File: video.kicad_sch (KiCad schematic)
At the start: 4 parts, among them J2 Board Interconnect Female, J2 Video Output Female, J3 Conn_02x08_Odd_Even

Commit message: move to samx4
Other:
- company: (none) -> Dragon Data
- title: (none) -> Dragon 32 CPU UK PAL
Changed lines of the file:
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@@
   (paper "A3")
   (title_block
+    (title "Dragon 32 CPU UK PAL")
     (date "2023-05-25")
     (rev "3.0")
-    (comment 2 "Reposition dram and buffer")
+    (company "Dragon Data")
+    (comment 1 "Modified by Julian Brown")
+    (comment 2 "SAMx4 by Ciaran Anscomb")
   )
   (no_connect (at 167.64 168.91))

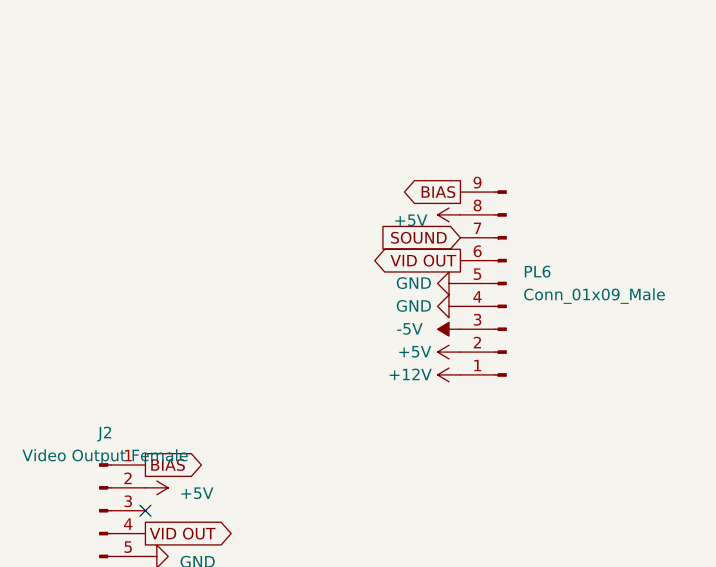
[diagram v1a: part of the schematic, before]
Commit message: serial wiring
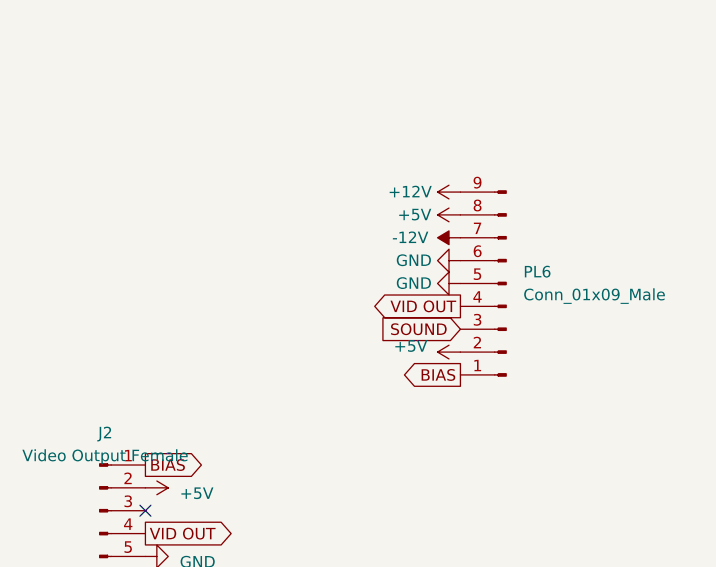
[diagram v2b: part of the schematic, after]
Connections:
- net +12V: now also PL6.9 (Pin_9); no longer PL6.1 (Pin_1)
- net -5V: no longer PL6.3 (Pin_3)
- net BIAS: now also PL6.1 (Pin_1); no longer PL6.9 (Pin_9)
- net GND: now also PL6.6 (Pin_6); no longer PL6.4 (Pin_4)
- net SOUND: now also PL6.3 (Pin_3); no longer PL6.7 (Pin_7)
- net VID OUT: now also PL6.4 (Pin_4); no longer PL6.6 (Pin_6)
- new net -12V: PL6.7 (Pin_7)
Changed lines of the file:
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@@
     )
   )
-  (global_label "VID OUT" (shape output) (at 202.6412 141.1224 180) (fields_autoplaced)
-    (effects (font (size 1.27 1.27)) (justify right))
-    (property "Intersheetrefs" "${INTERSHEET_REFS}" (at 193.0356 141.1224 0)
+  (global_label "VID OUT" (shape output) (at 202.6412 146.2024 180) (fields_autoplaced)
+    (effects (font (size 1.27 1.27)) (justify right))
+    (property "Intersheetrefs" "${INTERSHEET_REFS}" (at 193.0356 146.2024 0)
       (effects (font (size 1.27 1.27)) (justify right) hide)
     )
@@
     )
   )
-  (global_label "SOUND" (shape input) (at 202.6412 138.5824 180) (fields_autoplaced)
-    (effects (font (size 1.27 1.27)) (justify right))
-    (property "Intersheetrefs" "${INTERSHEET_REFS}" (at 193.9186 138.5824 0)
+  (global_label "SOUND" (shape input) (at 202.6412 148.7424 180) (fields_autoplaced)
+    (effects (font (size 1.27 1.27)) (justify right))
+    (property "Intersheetrefs" "${INTERSHEET_REFS}" (at 193.9186 148.7424 0)
       (effects (font (size 1.27 1.27)) (justify right) hide)
     )
@@
     )
   )
-  (global_label "BIAS" (shape output) (at 202.6412 133.5024 180) (fields_autoplaced)
-    (effects (font (size 1.27 1.27)) (justify right))
-    (property "Intersheetrefs" "${INTERSHEET_REFS}" (at 196.2167 133.5024 0)
+  (global_label "BIAS" (shape output) (at 202.6412 153.8224 180) (fields_autoplaced)
+    (effects (font (size 1.27 1.27)) (justify right))
+    (property "Intersheetrefs" "${INTERSHEET_REFS}" (at 196.2167 153.8224 0)
       (effects (font (size 1.27 1.27)) (justify right) hide)
     )
@@
     )
   )
-  (symbol (lib_id "power:GND") (at 202.6412 146.2024 270) (unit 1)
-    (in_bom yes) (on_board yes) (dnp no) (fields_autoplaced)
-    (property "Reference" "#PWR019" (at 196.2912 146.2024 0)
-      (effects (font (size 1.27 1.27)) hide)
-    )
-    (property "Value" "GND" (at 199.4662 146.2023 90)
+  (symbol (lib_id "power:GND") (at 202.6412 141.1224 270) (mirror x) (unit 1)
+    (in_bom yes) (on_board yes) (dnp no) (fields_autoplaced)
+    (property "Reference" "#PWR019" (at 196.2912 141.1224 0)
+      (effects (font (size 1.27 1.27)) hide)
+    )
+    (property "Value" "GND" (at 199.4662 141.1225 90)
       (effects (font (size 1.27 1.27)) (justify right))
     )
-    (property "Footprint" "" (at 202.6412 146.2024 0)
-      (effects (font (size 1.27 1.27)) hide)
-    )
-    (property "Datasheet" "" (at 202.6412 146.2024 0)
+    (property "Footprint" "" (at 202.6412 141.1224 0)
+      (effects (font (size 1.27 1.27)) hide)
+    )
+    (property "Datasheet" "" (at 202.6412 141.1224 0)
       (effects (font (size 1.27 1.27)) hide)
     )
@@
     )
   )
-  (symbol (lib_id "power:+5V") (at 202.6412 151.2824 90) (unit 1)
+  (symbol (lib_id "power:+5V") (at 202.6412 136.0424 90) (mirror x) (unit 1)
     (in_bom yes) (on_board yes) (dnp no)
-    (property "Reference" "#PWR0281" (at 206.4512 151.2824 0)
-      (effects (font (size 1.27 1.27)) hide)
-    )
-    (property "Value" "+5V" (at 195.6562 151.2824 90)
+    (property "Reference" "#PWR0281" (at 206.4512 136.0424 0)
+      (effects (font (size 1.27 1.27)) hide)
+    )
+    (property "Value" "+5V" (at 195.6562 136.0424 90)
       (effects (font (size 1.27 1.27)) (justify right))
     )
+    (property "Footprint" "" (at 202.6412 136.0424 0)
+      (effects (font (size 1.27 1.27)) hide)
+    )
+    (property "Datasheet" "" (at 202.6412 136.0424 0)
+      (effects (font (size 1.27 1.27)) hide)
+    )
+    (pin "1")
+    (instances
+      (project "Dragon32"
+        (path "/0c3dceba-7c95-4b3d-b590-0eb581444beb/d9dba8db-e731-4cb4-b2de-fefd65b288bc"
+          (reference "#PWR0281") (unit 1)
+        )
+      )
+    )
+  )
+  (symbol (lib_id "power:+5V") (at 202.6412 151.2824 90) (mirror x) (unit 1)
+    (in_bom yes) (on_board yes) (dnp no) (fields_autoplaced)
+    (property "Reference" "#PWR052" (at 206.4512 151.2824 0)
+      (effects (font (size 1.27 1.27)) hide)
+    )
+    (property "Value" "+5V" (at 198.9836 150.6474 90)
+      (effects (font (size 1.27 1.27)) (justify left))
+    )
     (property "Footprint" "" (at 202.6412 151.2824 0)
       (effects (font (size 1.27 1.27)) hide)
     )
     (property "Datasheet" "" (at 202.6412 151.2824 0)
-      (effects (font (size 1.27 1.27)) hide)
-    )
-    (pin "1")
-    (instances
-      (project "Dragon32"
-        (path "/0c3dceba-7c95-4b3d-b590-0eb581444beb/d9dba8db-e731-4cb4-b2de-fefd65b288bc"
-          (reference "#PWR0281") (unit 1)
-        )
-      )
-    )
-  )
-  (symbol (lib_id "power:+5V") (at 202.6412 136.0424 90) (unit 1)
-    (in_bom yes) (on_board yes) (dnp no) (fields_autoplaced)
-    (property "Reference" "#PWR052" (at 206.4512 136.0424 0)
-      (effects (font (size 1.27 1.27)) hide)
-    )
-    (property "Value" "+5V" (at 198.9836 136.6774 90)
-      (effects (font (size 1.27 1.27)) (justify left))
-    )
-    (property "Footprint" "" (at 202.6412 136.0424 0)
-      (effects (font (size 1.27 1.27)) hide)
-    )
-    (property "Datasheet" "" (at 202.6412 136.0424 0)
       (effects (font (size 1.27 1.27)) hide)
     )
@@
     )
   )
+  (symbol (lib_id "power:-12V") (at 202.6412 138.5824 90) (unit 1)
+    (in_bom yes) (on_board yes) (dnp no) (fields_autoplaced)
+    (property "Reference" "#PWR095" (at 200.1012 138.5824 0)
+      (effects (font (size 1.27 1.27)) hide)
+    )
+    (property "Value" "-12V" (at 199.0852 138.5824 90)
+      (effects (font (size 1.27 1.27)) (justify left))
+    )
+    (property "Footprint" "" (at 202.6412 138.5824 0)
+      (effects (font (size 1.27 1.27)) hide)
+    )
+    (property "Datasheet" "" (at 202.6412 138.5824 0)
+      (effects (font (size 1.27 1.27)) hide)
+    )
+    (pin "1")
+    (instances
+      (project "Dragon32"
+        (path "/0c3dceba-7c95-4b3d-b590-0eb581444beb/d9dba8db-e731-4cb4-b2de-fefd65b288bc"
+          (reference "#PWR095") (unit 1)
+        )
+      )
+    )
+  )
   (symbol (lib_id "power:GND") (at 137.1092 167.9448 90) (unit 1)
     (in_bom yes) (on_board yes) (dnp no) (fields_autoplaced)
@@
     )
   )
-  (symbol (lib_id "power:-5V") (at 202.6412 148.7424 90) (unit 1)
-    (in_bom yes) (on_board yes) (dnp no)
-    (property "Reference" "#PWR0282" (at 200.1012 148.7424 0)
-      (effects (font (size 1.27 1.27)) hide)
-    )
-    (property "Value" "-5V" (at 195.5292 148.7424 90)
-      (effects (font (size 1.27 1.27)) (justify right))
-    )
-    (property "Footprint" "" (at 202.6412 148.7424 0)
-      (effects (font (size 1.27 1.27)) hide)
-    )
-    (property "Datasheet" "" (at 202.6412 148.7424 0)
-      (effects (font (size 1.27 1.27)) hide)
-    )
-    (pin "1")
-    (instances
-      (project "Dragon32"
-        (path "/0c3dceba-7c95-4b3d-b590-0eb581444beb/d9dba8db-e731-4cb4-b2de-fefd65b288bc"
-          (reference "#PWR0282") (unit 1)
-        )
-      )
-    )
-  )
-  (symbol (lib_id "power:GND") (at 202.6412 143.6624 270) (unit 1)
+  (symbol (lib_id "power:GND") (at 202.6412 143.6624 270) (mirror x) (unit 1)
     (in_bom yes) (on_board yes) (dnp no) (fields_autoplaced)
     (property "Reference" "#PWR018" (at 196.2912 143.6624 0)
       (effects (font (size 1.27 1.27)) hide)
     )
-    (property "Value" "GND" (at 199.4662 143.6623 90)
+    (property "Value" "GND" (at 199.4662 143.6625 90)
       (effects (font (size 1.27 1.27)) (justify right))
     )
@@
     )
   )
-  (symbol (lib_id "power:+12V") (at 202.6412 153.8224 90) (unit 1)
-    (in_bom yes) (on_board yes) (dnp no) (fields_autoplaced)
-    (property "Reference" "#PWR022" (at 206.4512 153.8224 0)
-      (effects (font (size 1.27 1.27)) hide)
-    )
-    (property "Value" "+12V" (at 199.4662 153.8223 90)
+  (symbol (lib_id "power:+12V") (at 202.6412 133.5024 90) (mirror x) (unit 1)
+    (in_bom yes) (on_board yes) (dnp no) (fields_autoplaced)
+    (property "Reference" "#PWR022" (at 206.4512 133.5024 0)
+      (effects (font (size 1.27 1.27)) hide)
+    )
+    (property "Value" "+12V" (at 199.4662 133.5025 90)
       (effects (font (size 1.27 1.27)) (justify left))
     )
-    (property "Footprint" "" (at 202.6412 153.8224 0)
-      (effects (font (size 1.27 1.27)) hide)
-    )
-    (property "Datasheet" "" (at 202.6412 153.8224 0)
-      (effects (font (size 1.27 1.27)) hide)
-    )
+    (property "Footprint" "" (at 202.6412 133.5024 0)
+      (effects (font (size 1.27 1.27)) hide)
+    )
+    (property "Datasheet" "" (at 202.6412 133.5024 0)
+      (effects (font (size 1.27 1.27)) hide)
+    )
